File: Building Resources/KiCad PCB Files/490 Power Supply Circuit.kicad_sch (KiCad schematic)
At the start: 24 parts, among them J1 Screw_Terminal_01x10, J2 Conn_01x12_Pin, U1 LM2596T-3.3, U3 ESP32-DEVKITC-32D

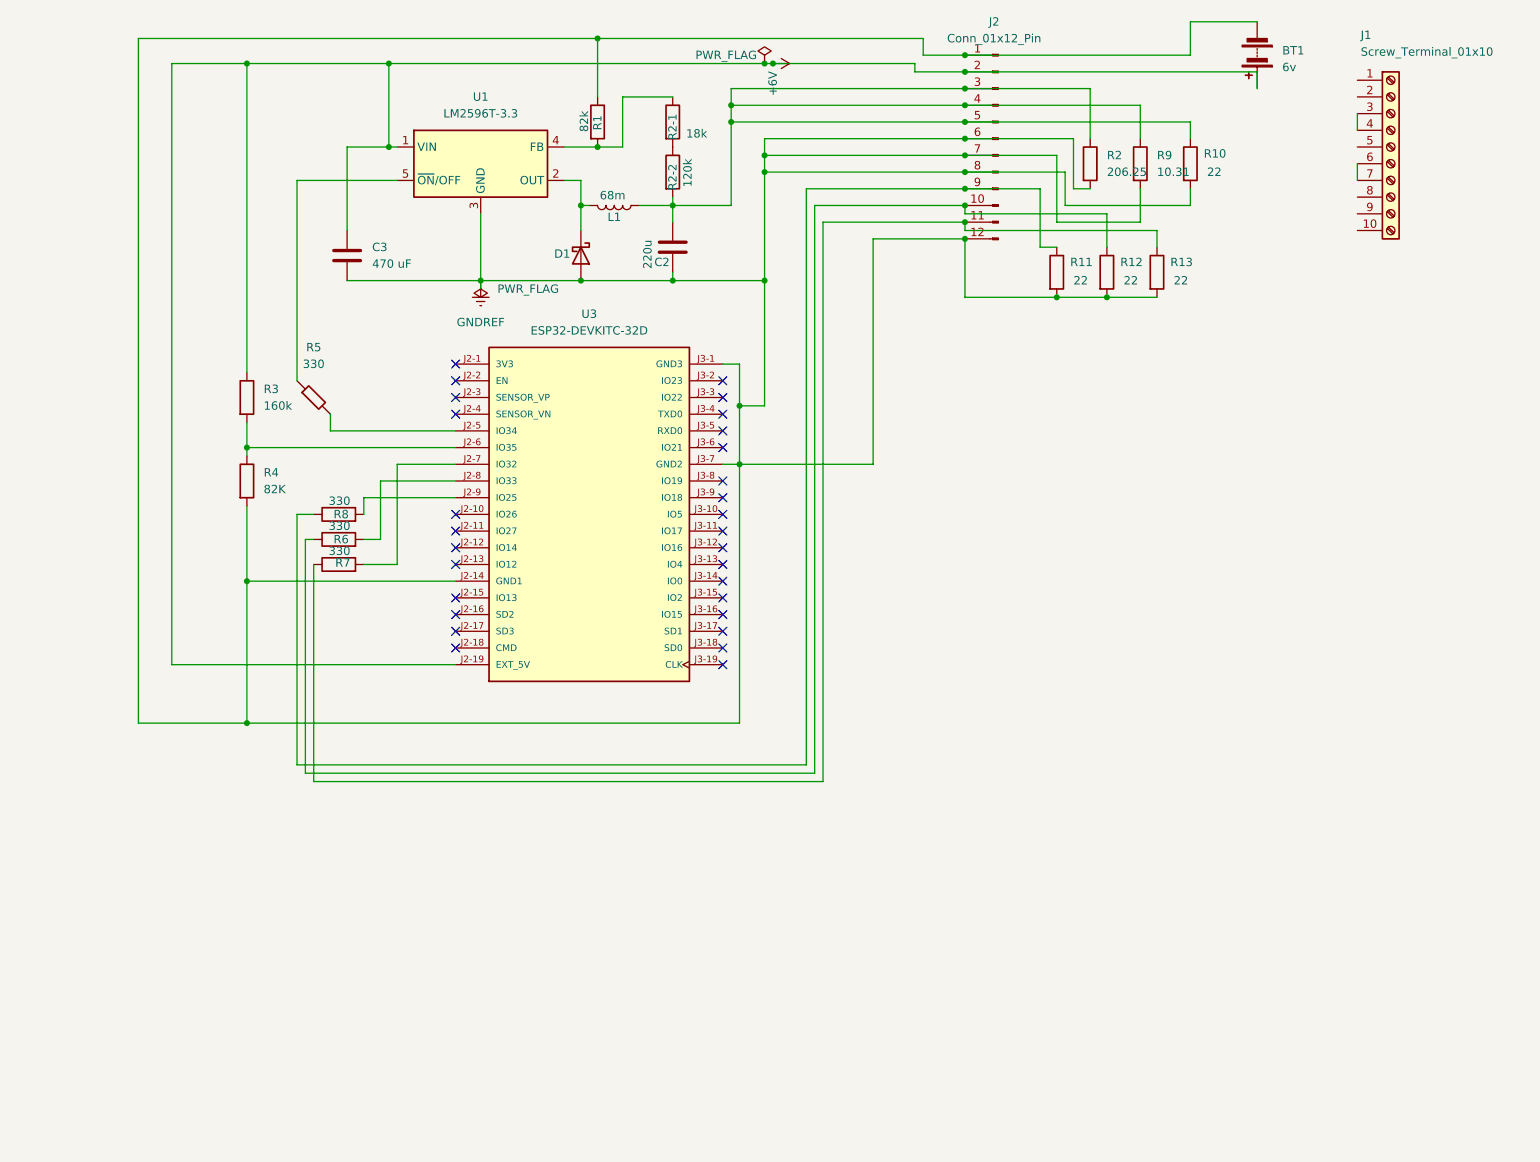
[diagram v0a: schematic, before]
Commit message: Upload new KiCad Files.
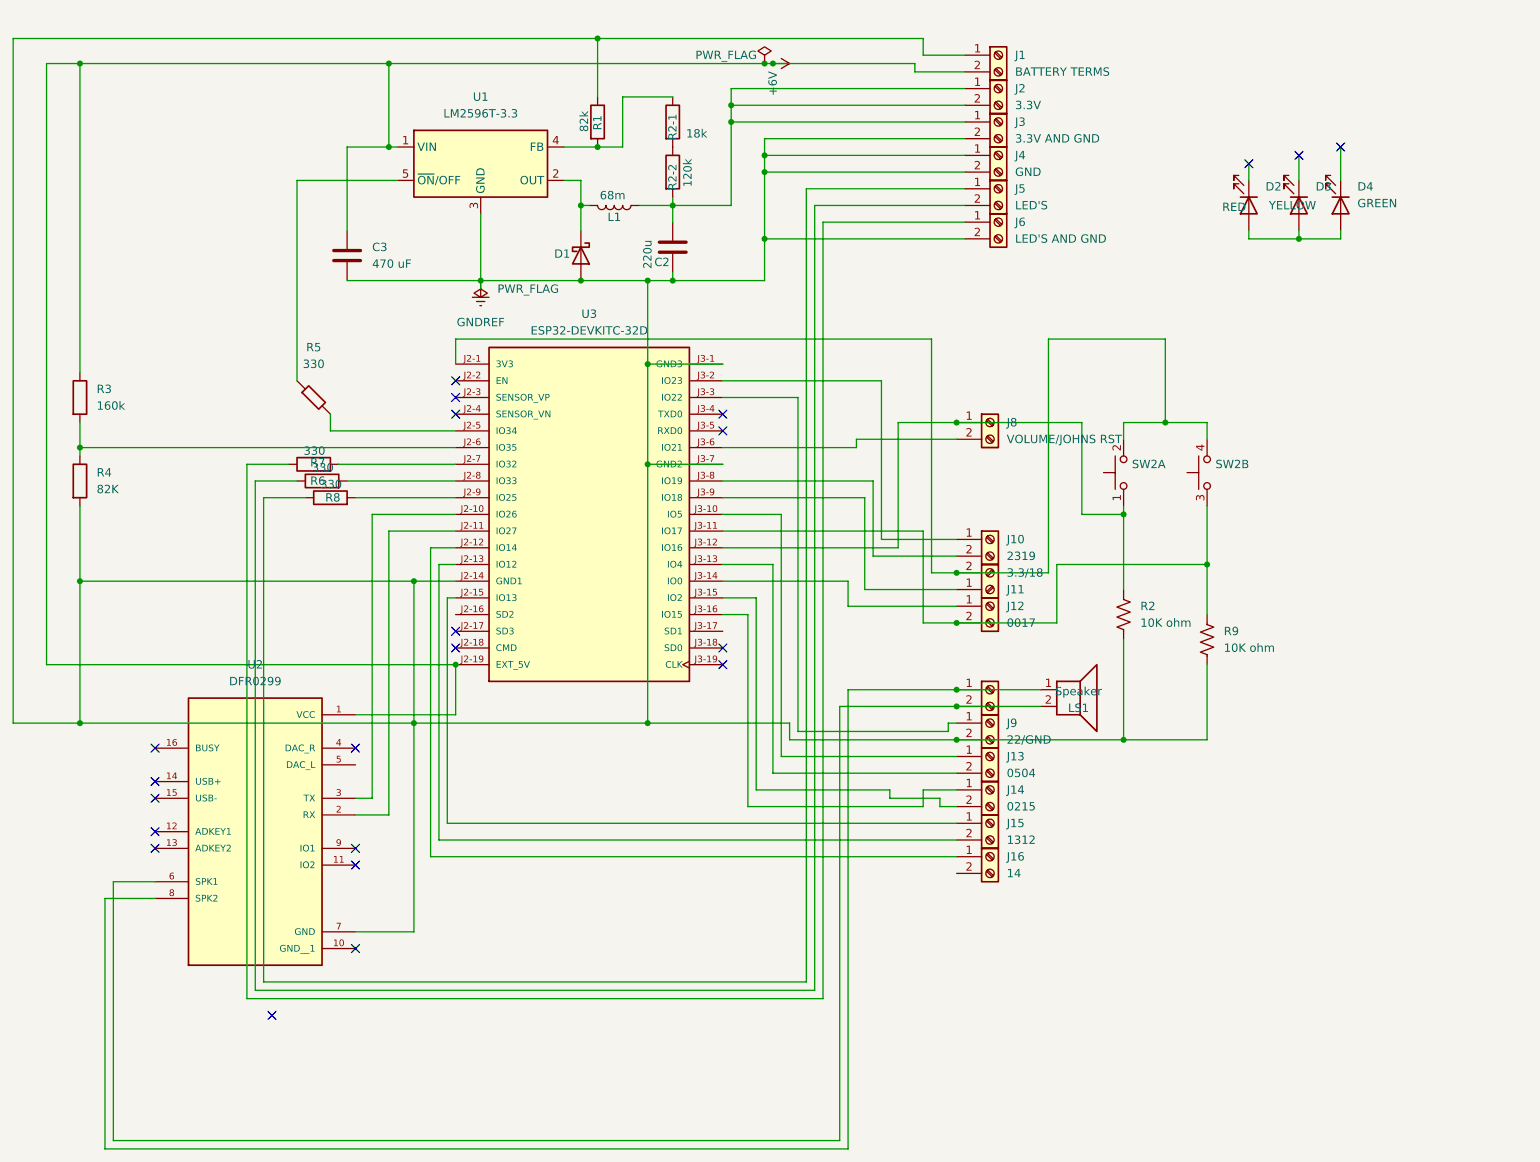
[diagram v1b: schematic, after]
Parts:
- removed BT1: 6v, symbol Device:Battery
- removed J1: Screw_Terminal_01x10, TerminalBlock:TerminalBlock_MaiXu_MX126-5.0-10P_1x10_P5.00mm, symbol Connector:Screw_Terminal_01x10
- removed J2: Conn_01x12_Pin, symbol Connector:Conn_01x12_Pin
- removed R10, R11, R12, R13: 22, symbol Device:R
- removed R2: 206.25, symbol Device:R
- removed R9: 10.31, symbol Device:R
- added D2: RED, LED_THT:LED_D4.0mm, symbol Device:LED
- added D3: YELLOW, LED_THT:LED_D4.0mm, symbol Device:LED
- added D4: GREEN, LED_THT:LED_D4.0mm, symbol Device:LED
- added J1: BATTERY TERMS, TerminalBlock_4Ucon:TerminalBlock_4Ucon_1x02_P3.50mm_Vertical, symbol Connector:Screw_Terminal_01x02
- added J10: 2319, TerminalBlock_4Ucon:TerminalBlock_4Ucon_1x02_P3.50mm_Vertical, symbol Connector:Screw_Terminal_01x02
- added J11: 3.3/18, TerminalBlock_4Ucon:TerminalBlock_4Ucon_1x02_P3.50mm_Vertical, symbol Connector:Screw_Terminal_01x02
- added J12: 0017, TerminalBlock_4Ucon:TerminalBlock_4Ucon_1x02_P3.50mm_Vertical, symbol Connector:Screw_Terminal_01x02
- added J13: 0504, TerminalBlock_4Ucon:TerminalBlock_4Ucon_1x02_P3.50mm_Vertical, symbol Connector:Screw_Terminal_01x02
- added J14: 0215, TerminalBlock_4Ucon:TerminalBlock_4Ucon_1x02_P3.50mm_Vertical, symbol Connector:Screw_Terminal_01x02
- added J15: 1312, TerminalBlock_4Ucon:TerminalBlock_4Ucon_1x02_P3.50mm_Vertical, symbol Connector:Screw_Terminal_01x02
- added J16: 14, TerminalBlock_4Ucon:TerminalBlock_4Ucon_1x02_P3.50mm_Vertical, symbol Connector:Screw_Terminal_01x02
- added J2: 3.3V, TerminalBlock_4Ucon:TerminalBlock_4Ucon_1x02_P3.50mm_Vertical, symbol Connector:Screw_Terminal_01x02
- added J3: 3.3V AND GND, TerminalBlock_4Ucon:TerminalBlock_4Ucon_1x02_P3.50mm_Vertical, symbol Connector:Screw_Terminal_01x02
- added J4: GND, TerminalBlock_4Ucon:TerminalBlock_4Ucon_1x02_P3.50mm_Vertical, symbol Connector:Screw_Terminal_01x02
- added J5: LED'S, TerminalBlock_4Ucon:TerminalBlock_4Ucon_1x02_P3.50mm_Vertical, symbol Connector:Screw_Terminal_01x02
- added J6: LED'S AND GND, TerminalBlock_4Ucon:TerminalBlock_4Ucon_1x02_P3.50mm_Vertical, symbol Connector:Screw_Terminal_01x02
- added J7: SPEAKER, TerminalBlock_4Ucon:TerminalBlock_4Ucon_1x02_P3.50mm_Vertical, symbol Connector:Screw_Terminal_01x02
- added J8: VOLUME/JOHNS RST, TerminalBlock_4Ucon:TerminalBlock_4Ucon_1x02_P3.50mm_Vertical, symbol Connector:Screw_Terminal_01x02
- added J9: 22/GND, TerminalBlock_4Ucon:TerminalBlock_4Ucon_1x02_P3.50mm_Vertical, symbol Connector:Screw_Terminal_01x02
- added LS1: Speaker, symbol Device:Speaker
- added R2, R9: 10K ohm, symbol Device:R_US
- added SW2: SW_Push_Dual_x2, symbol Switch:SW_Push_Dual_x2
- added U2: DFR0299, DFR0299:DFR0299, symbol DFR0299:DFR0299
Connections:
- net +6V: now also J1.2 (Pin_2), U2.1 (VCC)
- net GNDREF: now also J1.1 (Pin_1), J3.2 (Pin_2), J4.1 (Pin_1), J4.2 (Pin_2), J6.2 (Pin_2), J9.2 (Pin_2), R2.2, R9.2, U2.7 (GND)
- net at R7.1: now also J6.1 (Pin_1)
- net at R6.1: now also J5.2 (Pin_2)
- net at C2.1, L1.1, R2-2.2: now also J2.1 (Pin_1), J2.2 (Pin_2), J3.1 (Pin_1)
- net at R8.1: now also J5.1 (Pin_1)
- net at U3.J2-1 (3V3): now also J11.2 (Pin_2), SW2.2 (D), SW2.4 (D)
- net at U3.J2-10 (IO26): now also U2.3 (TX)
- net at U3.J2-11 (IO27): now also U2.2 (RX)
- net at U3.J2-12 (IO14): now also J16.1 (Pin_1)
- net at U3.J2-13 (IO12): now also J15.2 (Pin_2)
- net at U3.J2-15 (IO13): now also J15.1 (Pin_1)
- net at U3.J3-10 (IO5): now also J13.1 (Pin_1)
- net at U3.J3-11 (IO17): now also J12.2 (Pin_2), R9.1, SW2.3 (C)
- net at U3.J3-12 (IO16): now also J8.1 (Pin_1), R2.1, SW2.1 (C)
- net at U3.J3-13 (IO4): now also J13.2 (Pin_2)
- net at U3.J3-14 (IO0): now also J12.1 (Pin_1)
- net at U3.J3-15 (IO2): now also J14.2 (Pin_2)
- net at U3.J3-16 (IO15): now also J14.1 (Pin_1)
- net at U3.J3-2 (IO23): now also J10.1 (Pin_1)
- net at U3.J3-3 (IO22): now also J9.1 (Pin_1)
- net at U3.J3-6 (IO21): now also J8.2 (Pin_2)
- net at U3.J3-8 (IO19): now also J10.2 (Pin_2)
- net at U3.J3-9 (IO18): now also J11.1 (Pin_1)
- new net: D2.2 (A), D3.2 (A), D4.2 (A)
- new net: J7.1 (Pin_1), LS1.1, U2.8 (SPK2)
- new net: J7.2 (Pin_2), LS1.2, U2.6 (SPK1)
- no-connect marks 29 -> 22
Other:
- moved on the sheet: R3, R4, R6, R7, R8
